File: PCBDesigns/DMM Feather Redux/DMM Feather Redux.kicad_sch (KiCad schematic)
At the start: 50 parts, among them J10 I_Input, J14 Barrel_Jack, J2 Conn_01x03_Pin, J3 Conn_01x04_MountingPin, J7 Barrel_Jack, Q2 AO3400A MOSFET, Q8 AO3400A MOSFET, SW3 SW_SPDT, U1 ISO1644DWR, U10 LM4040DBZ-2.5, U13 ISO1540, U14 0305 DCDC Converter, U3 ADS1115IDGS, U4 ADuM1410, U5 LM317_TO-220, U6 LM4040DBZ-5, U7 IX4426N, U8 MAX1683

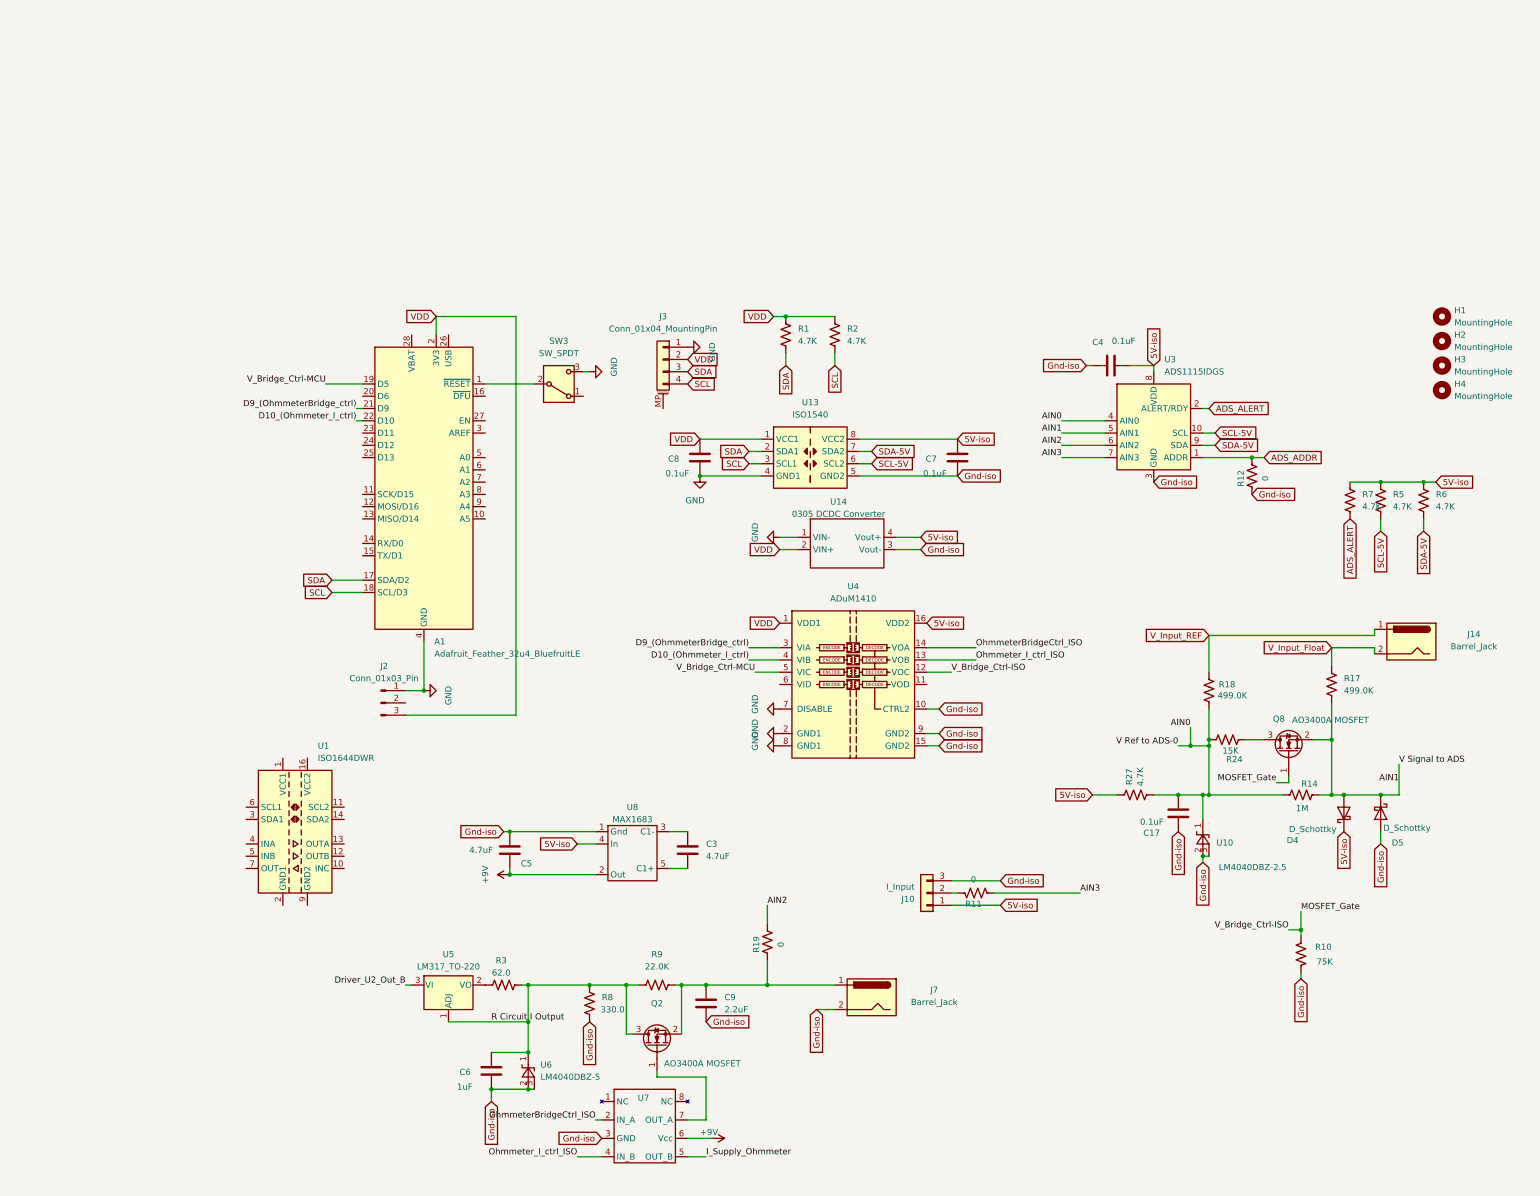
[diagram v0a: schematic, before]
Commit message: Work on different PCBs. Mostly.
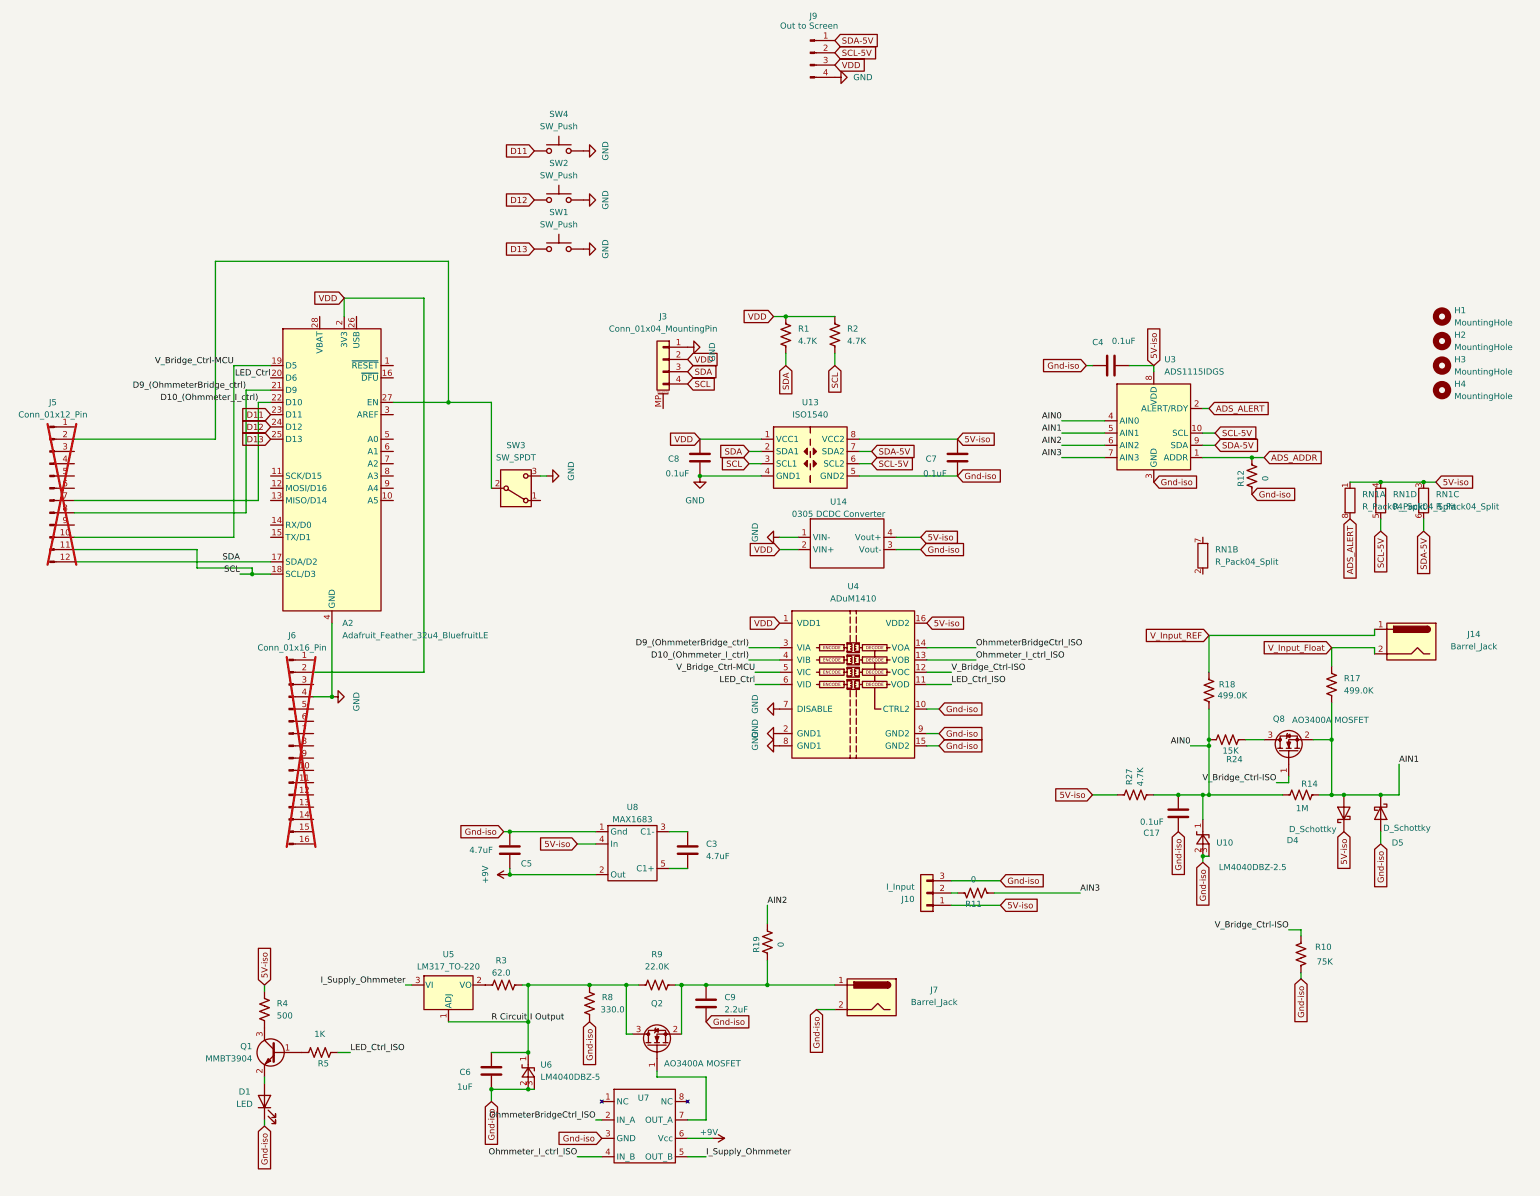
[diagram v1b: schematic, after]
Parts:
- removed A1: Adafruit_Feather_32u4_BluefruitLE, Module:Adafruit_Feather_WithMountingHoles, symbol MCU_Module:Adafruit_Feather_32u4_BluefruitLE
- removed J2: Conn_01x03_Pin, Connector_PinHeader_2.54mm:PinHeader_1x03_P2.54mm_Vertical, symbol Connector:Conn_01x03_Pin
- removed R6, R7: 4.7K, Resistor_SMD:R_0805_2012Metric_Pad1.20x1.40mm_HandSolder, symbol Device:R_US
- removed U1: ISO1644DWR, Package_SO:SOIC-16W_7.5x10.3mm_P1.27mm, symbol Isolator:ISO1644DWR
- added A2: Adafruit_Feather_32u4_BluefruitLE, Module:Adafruit_Feather_WithMountingHoles, symbol MCU_Module:Adafruit_Feather_32u4_BluefruitLE
- added D1: LED, LED_SMD:LED_Luminus_MP-3030-1100_3.0x3.0mm, symbol Device:LED
- added J5: Conn_01x12_Pin, Connector_PinSocket_2.54mm:PinSocket_1x12_P2.54mm_Vertical, symbol Connector:Conn_01x12_Pin
- added J6: Conn_01x16_Pin, Connector_PinSocket_2.54mm:PinSocket_1x16_P2.54mm_Vertical, symbol Connector:Conn_01x16_Pin
- added J9: Out to Screen, Connector_PinSocket_2.54mm:PinSocket_1x04_P2.54mm_Vertical, symbol Connector:Conn_01x04_Pin
- added Q1: MMBT3904, Package_TO_SOT_SMD:SOT-23, symbol Transistor_BJT:MMBT3904
- added R4: 500, Resistor_SMD:R_0805_2012Metric_Pad1.20x1.40mm_HandSolder, symbol Device:R_US
- added RN1: R_Pack04_Split, Resistor_SMD:R_Array_Convex_4x0603, symbol Device:R_Pack04_Split
- added SW1, SW2, SW4: SW_Push, Button_Switch_SMD:SW_SPST_CK_RS282G05A3, symbol Switch:SW_Push
- C17, C4, C7, C8: footprint Capacitor_SMD:C_0805_2012Metric_Pad1.18x1.45mm_HandSolder -> Capacitor_SMD:C_0603_1608Metric
- R1, R10, R11, R12, R19, R2, R27: footprint Resistor_SMD:R_0805_2012Metric_Pad1.20x1.40mm_HandSolder -> Resistor_SMD:R_0603_1608Metric
- R5: value 4.7K -> 1K; footprint Resistor_SMD:R_0805_2012Metric_Pad1.20x1.40mm_HandSolder -> Resistor_SMD:R_0603_1608Metric; Function (none) -> I limit for Q1
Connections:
- net Driver_U2_Out_B is gone; now on net I_Supply_Ohmmeter: U5.3 (VI)
- net 5V-iso: now also R4.2, RN1.1 (R1.1), RN1.3 (R3.1), RN1.4 (R4.1); no longer R5.1
- net ADS_ALERT: now also RN1.8 (R1.2)
- net D10_(Ohmmeter_I_ctrl): now also A2.22 (D10), J5.7 (Pin_7)
- net D9_(OhmmeterBridge_ctrl): now also A2.21 (D9), J5.8 (Pin_8)
- net GND: now also A2.4 (GND), J6.4 (Pin_4), J9.4 (Pin_4), SW1.2, SW2.2, SW4.2
- net Gnd-iso: now also D1.1 (K)
- net SCL: now also A2.18 (SCL/D3), J5.11 (Pin_11)
- net SCL-5V: now also J9.2 (Pin_2), RN1.5 (R4.2); no longer R5.2
- net SDA: now also A2.17 (SDA/D2), J5.12 (Pin_12)
- net SDA-5V: now also J9.1 (Pin_1), RN1.6 (R3.2)
- net VDD: now also A2.2 (3V3), J6.2 (Pin_2), J9.3 (Pin_3)
- net V_Bridge_Ctrl-MCU: now also A2.19 (D5), J5.10 (Pin_10)
- net LED_Ctrl_ISO: now reaches U4.11 (VOD)
- net LED_Ctrl_ISO: now also R5.1
- net LED_Ctrl: now reaches U4.6 (VID)
- net LED_Ctrl: now also A2.20 (D6)
- net at SW3.2 (B): now also A2.27 (EN), J5.2 (Pin_2)
- net MOSFET_Gate renamed V_Bridge_Ctrl-ISO
- new net: Q1.3 (C), R4.1
- new net: Q1.1 (B), R5.2
- new net: D1.2 (A), Q1.2 (E)
- new net D11: A2.23 (D11), SW4.1
- new net D12: A2.24 (D12), SW2.1
- new net D13: A2.25 (D13), SW1.1
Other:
- moved on the sheet: SW3
